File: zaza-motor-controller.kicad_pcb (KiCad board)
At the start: 2 copper layers, 53 x 60 mm, 74 parts, among them J1 VIN, J2 VIN, J3 CONN_02X05, J4 CONN_02X01, J5 GS3, Q1 BC337, Q10 BC327, Q11 BC337, Q12 BC337, Q2 BC337, Q3 BC327, Q4 BC337, Q5 IXTA220, Q6 IXTA220, Q7 IXTA220, Q8 IXTA220, Q9 BC337, U1 74HC00, U2 74HC00, U3 LM358, U4 LM555N

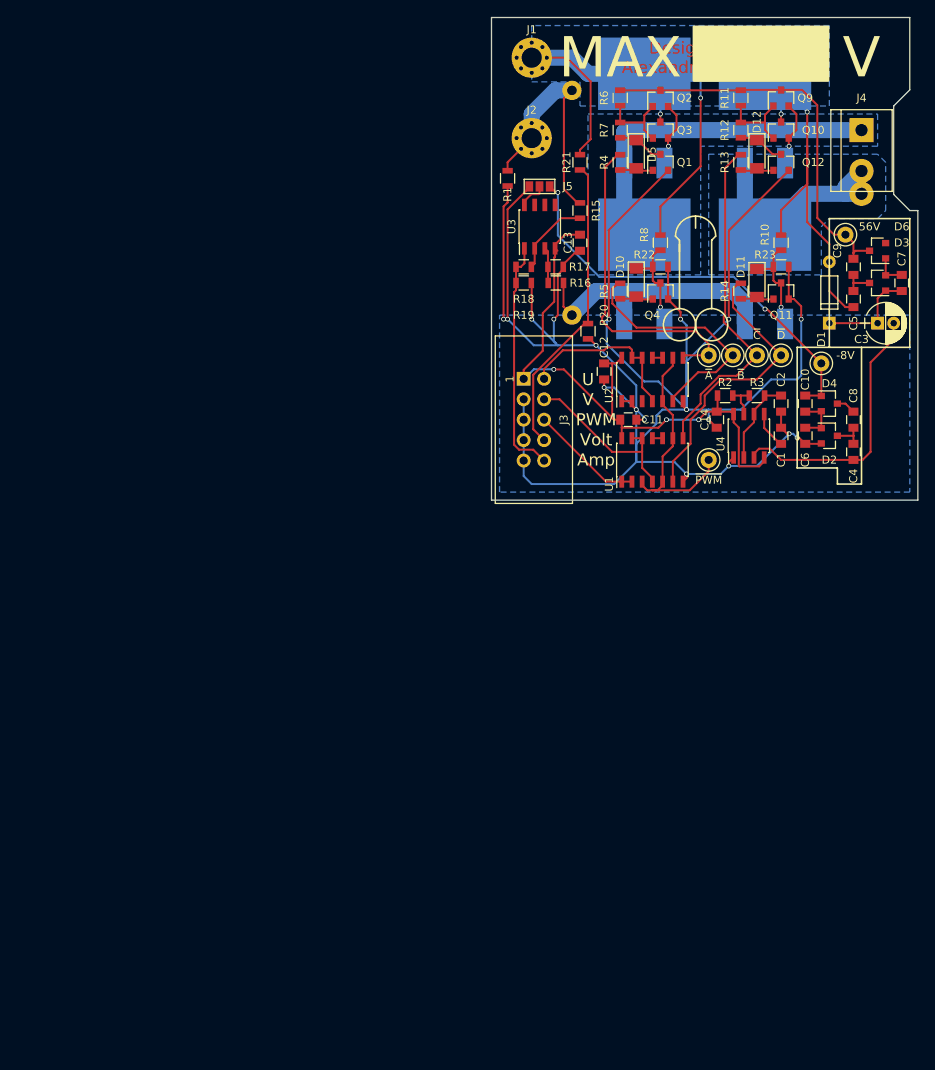
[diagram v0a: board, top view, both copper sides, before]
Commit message: Rev1 dev
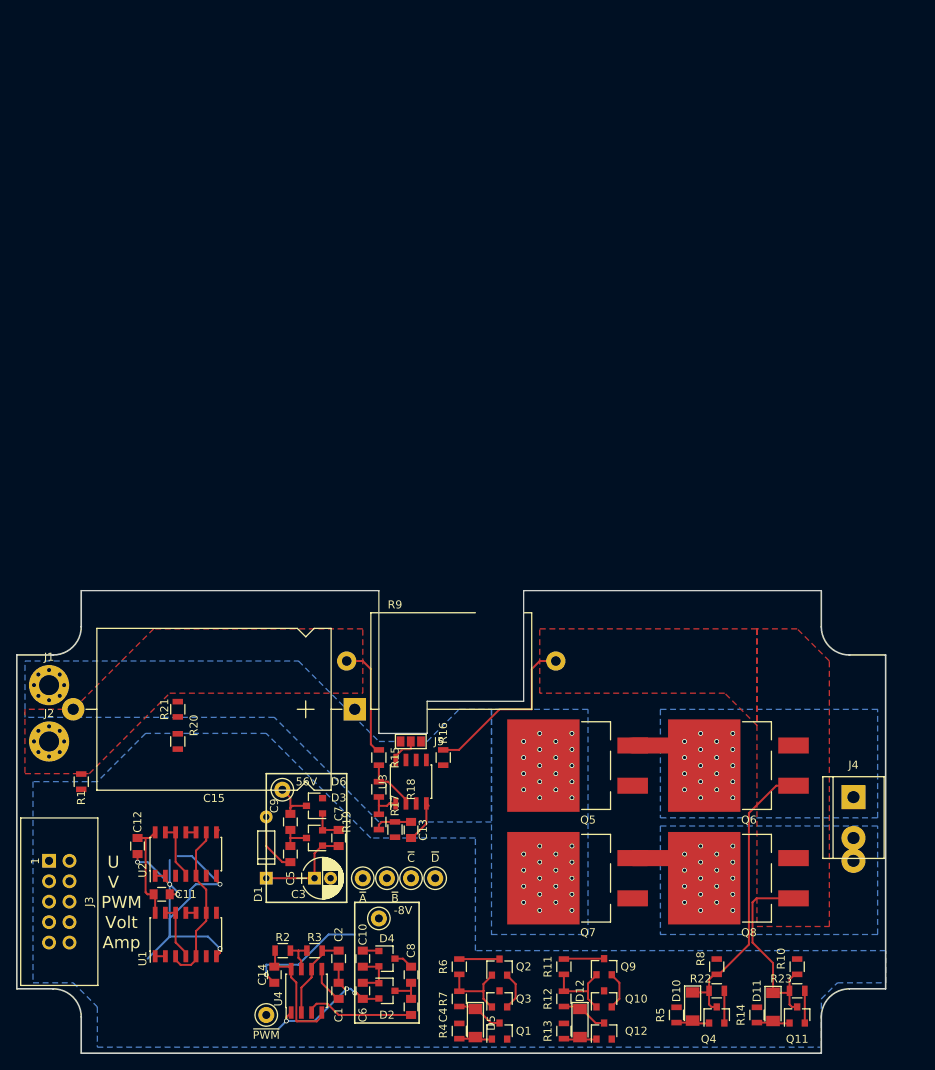
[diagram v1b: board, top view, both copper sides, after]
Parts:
- added C15: CP, Capacitors_THT:CP_Axial_L29.0mm_D20.0mm_P35.00mm_Horizontal, F.Cu at (83.0, 146.0)
- Q5, Q6, Q7, Q8, R9: moved to F.Cu
- moved D12 110.2 mm to (111.0, 185.0)
- moved Q10 110.2 mm to (114.0, 182.0)
- moved Q12 110.2 mm to (114.0, 186.0)
- moved Q9 110.2 mm to (114.0, 178.0)
- moved R11 110.2 mm to (109.0, 178.0)
- moved R12 110.2 mm to (109.0, 182.0)
- moved R13 110.2 mm to (109.0, 186.0)
- moved Q2 109.8 mm to (101.0, 178.1)
- moved D5 109.8 mm to (98.0, 185.0)
- moved Q1 109.8 mm to (101.0, 186.0)
- moved Q3 109.8 mm to (101.0, 182.0)
- moved R4 109.8 mm to (96.0, 186.0)
- moved R6 109.8 mm to (96.0, 178.0)
- moved R7 109.8 mm to (96.0, 182.0)
- moved J1 98.4 mm to (45.0, 143.0)
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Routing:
- net GND: track 293.1 -> 99.7 mm, vias 18 -> 9
- net +48V: track 137.1 -> 69.9 mm, vias 4 -> 36
- net VEE: track 52.1 -> 2.02 mm, vias 2 -> 0
- net +5V: track 77.7 -> 34.4 mm, vias 3 -> 0
- net /~C: track 43.1 -> 0.30 mm
- net /~A: track 41.0 -> 0.72 mm
- net /V_SENSE: track 37.5 -> 0.00 mm
- net /~D: track 35.9 -> 0.30 mm
- net HT: track 49.5 -> 15.8 mm
- net /~B: track 30.8 -> 0.75 mm
- net /I_SENSE: track 29.8 -> 4.97 mm
- net Net-(D10-Pad1): track 13.2 -> 36.8 mm, vias 1 -> 0
- net /PUMP_OSC: track 34.0 -> 14.3 mm
- net /M+: track 43.4 -> 24.8 mm, vias 0 -> 18
- net GNDPWR: track 29.9 -> 14.1 mm
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- added copper zone on F.Cu, net GNDPWR
- added copper zone on F.Cu, net Net-(Q6-Pad3)
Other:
- board size 53 x 60 mm -> 108 x 57.5 mm
- board text removed: "Designed by Alexandru Gagniuc"
- board text removed: "MAX"
